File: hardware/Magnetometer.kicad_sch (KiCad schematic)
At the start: 4 parts, among them IC2 BMM350

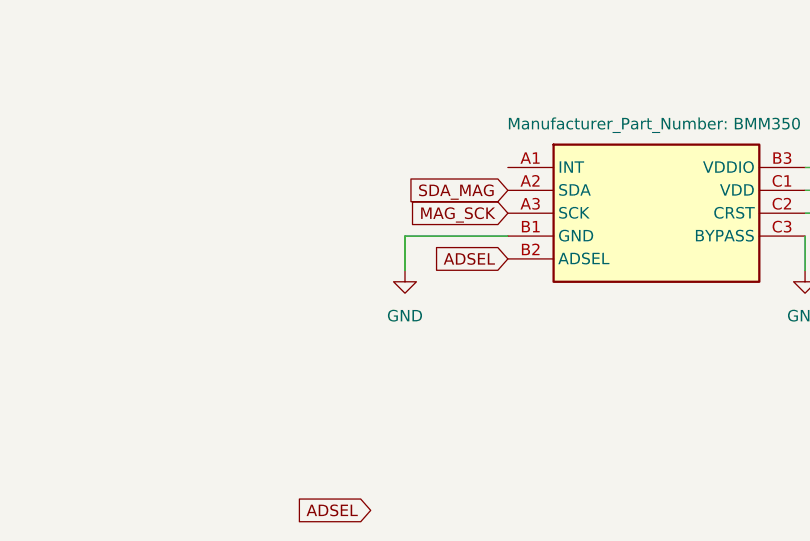
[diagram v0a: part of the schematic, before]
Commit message: fixed electrical rules
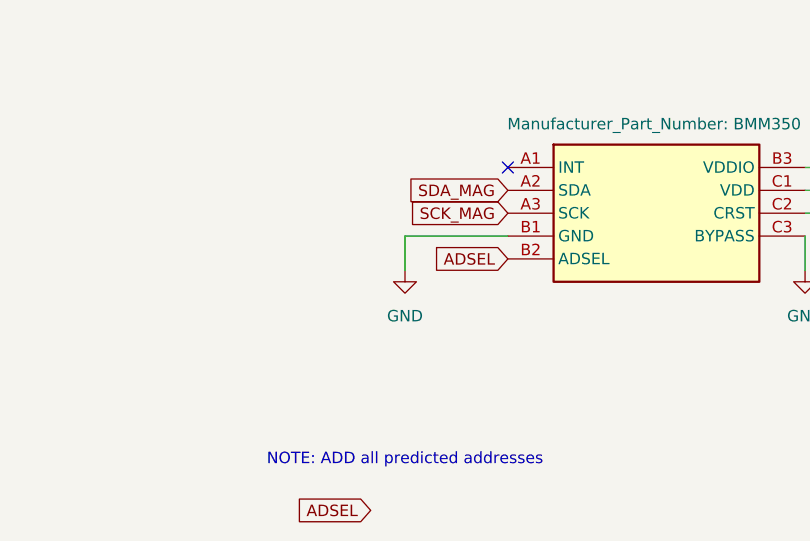
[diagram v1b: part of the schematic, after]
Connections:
- net MAG_SCK renamed SCK_MAG
- no-connect marks 0 -> 1
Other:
- note added: "NOTE: ADD all predicted addresses"
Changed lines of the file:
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@@
 	(generator_version "10.0")
 	(paper "A4")
+	(text "NOTE: ADD all predicted addresses\n"
+		(exclude_from_sim no)
+		(at 107.95 96.012 0)
+		(effects
+			(font
+				(size 1.27 1.27)
+			)
+		)
+	)
 	(junction
 		(at 177.8 63.5)
@@
 		(diameter 0)
 		(color 0 0 0 0)
+	)
+	(no_connect
+		(at 119.38 63.5)
 	)
 	(wire
@@
 		)
 	)
-	(global_label "MAG_SCK"
+	(global_label "SCK_MAG"
 		(shape input)
 		(at 119.38 68.58 180)
